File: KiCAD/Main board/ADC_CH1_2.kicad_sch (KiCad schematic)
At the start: 31 parts, among them U27 PCM1804, U5 OPA1632DR, U6 LM4562

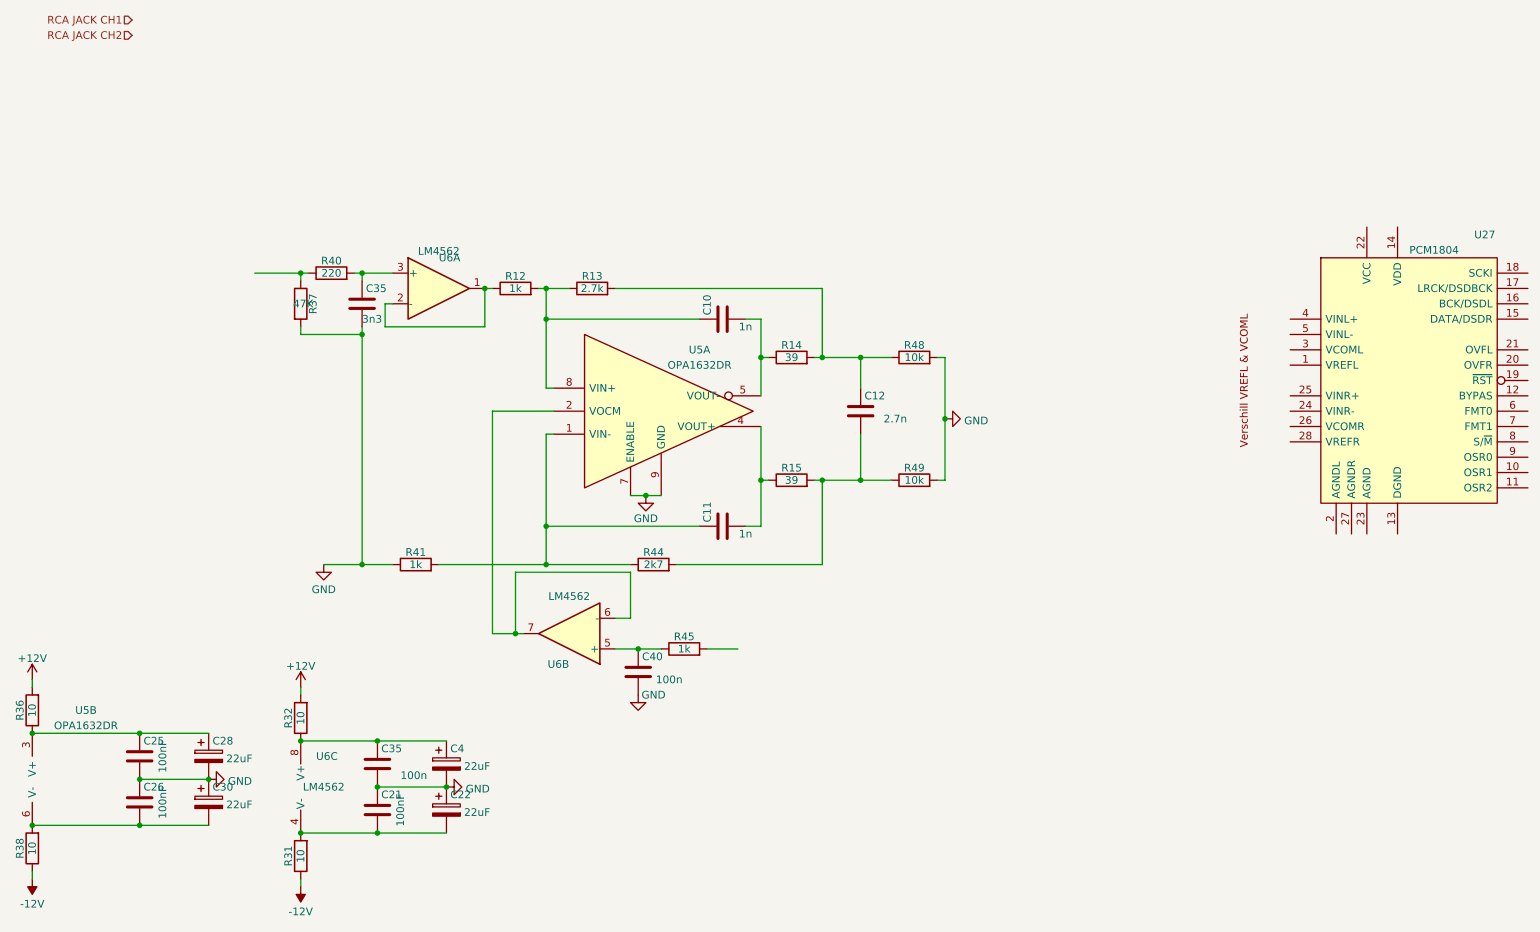
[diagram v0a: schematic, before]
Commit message: Worked on main board SCH
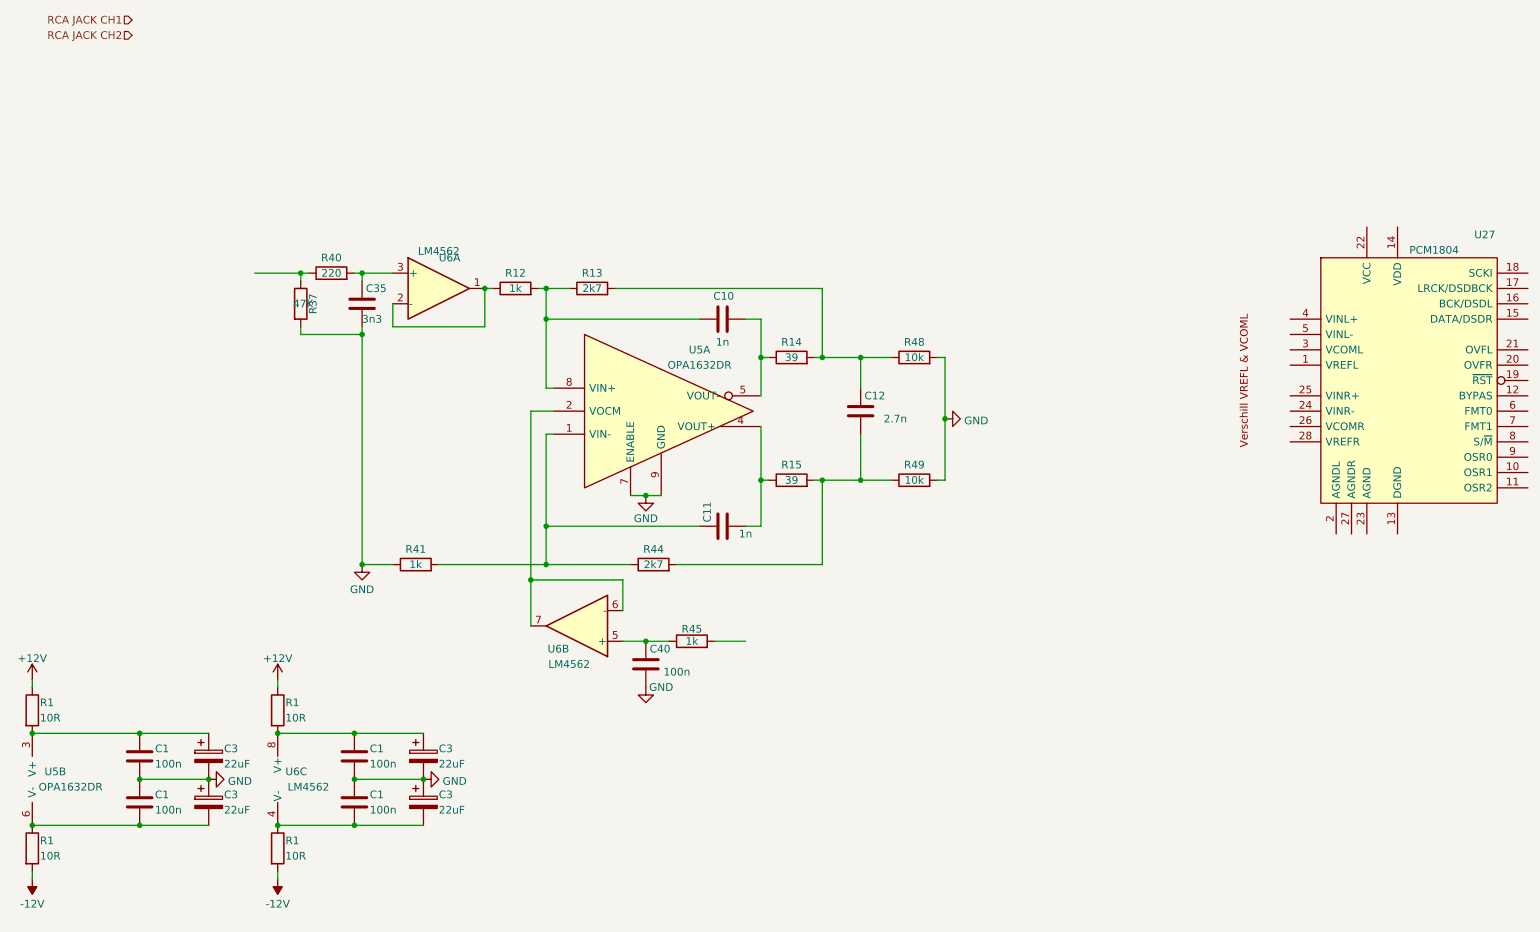
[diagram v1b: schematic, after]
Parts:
- removed C21, C25, C26: 100nF, symbol Device:C
- removed C22, C28, C30, C4: 22uF, symbol Device:C_Polarized
- removed C35: 100n, symbol Device:C
- removed R31, R32, R36, R38: 10, symbol Device:R
- added C1 (x4): 100n, Capacitor_SMD:C_0402_1005Metric, symbol Device:C
- added C3 (x4): 22uF, Capacitor_THT:CP_Radial_D5.0mm_P2.00mm, symbol Device:C_Polarized
- added R1 (x4): 10R, Resistor_SMD:R_0805_2012Metric, symbol Device:R
- R13: value 2.7k -> 2k7
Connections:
- net +12V: now also R1.1, R1.1
- net -12V: now also R1.2, R1.2
- net GND: now also C1.1, C1.1, C1.2, C1.2, C3.1, C3.1, C3.2, C3.2
- net at U6.8 (V+): now also C1.1, C3.1, R1.2
- net at U5.3 (V+): now also C1.1, C3.1, R1.2
- net at U6.4 (V-): now also C1.2, C3.2, R1.1
- net at U5.6 (V-): now also C1.2, C3.2, R1.1
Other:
- moved on the sheet: C40, R45, U6B, U6C
